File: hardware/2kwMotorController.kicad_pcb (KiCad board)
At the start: 4 copper layers, 170 x 98.5 mm, 415 parts, among them M3 MOUNTING_HOLE, M6 MOUNTING_HOLE, P1 CONN_01X02, P10 CONN_01_BRK, P11 CONN_01_M+, P12 CONN_01_M-, P13 CONN_01X02, P14 CONN_01X02, P15 CONN_01X04, P2 CONN_01X04, P3 CONN_01X09, P4 CONN_02X05, P5 CONN_01X03_UART, P6 CONN_01X03, P7 CONN_01X05, P8 CONN_01_V+, P9 CONN_01_V-, Q1 DMG4712SSS, Q10 PSMN021-100, Q2 DMG4712SSS, Q3 IRFP4468, Q5 IRFP4468, Q6 IRFP4468, Q7 IRFP4468, Q8 IRFP4468, Q9 IRFP4468, SW2 SW_PUSH, U1 LM358A, U10 MCP1501T-30E, U11 PDM1-S12-S3, U12 MIC5225-5.0, U13 TM4C1294KCPDT, U14 SN74LVCH2T45, U15 SN65HVD231D, U16 Si8045AA, U17 MIC4127, U18 MIC4127, U19 UCC27211, U2 LAH-100P, U20 Si8045AA, U21 74LVC1G17, U22 SN74LVCH2T45, U3 LOC110, U4 MCP6001, U5 ADA4805-1, U6 UCC27211, U7 MIC5225-5.0, U8 LT3471, U9 R-78E3.3-0.5, Y1 NX5032GA

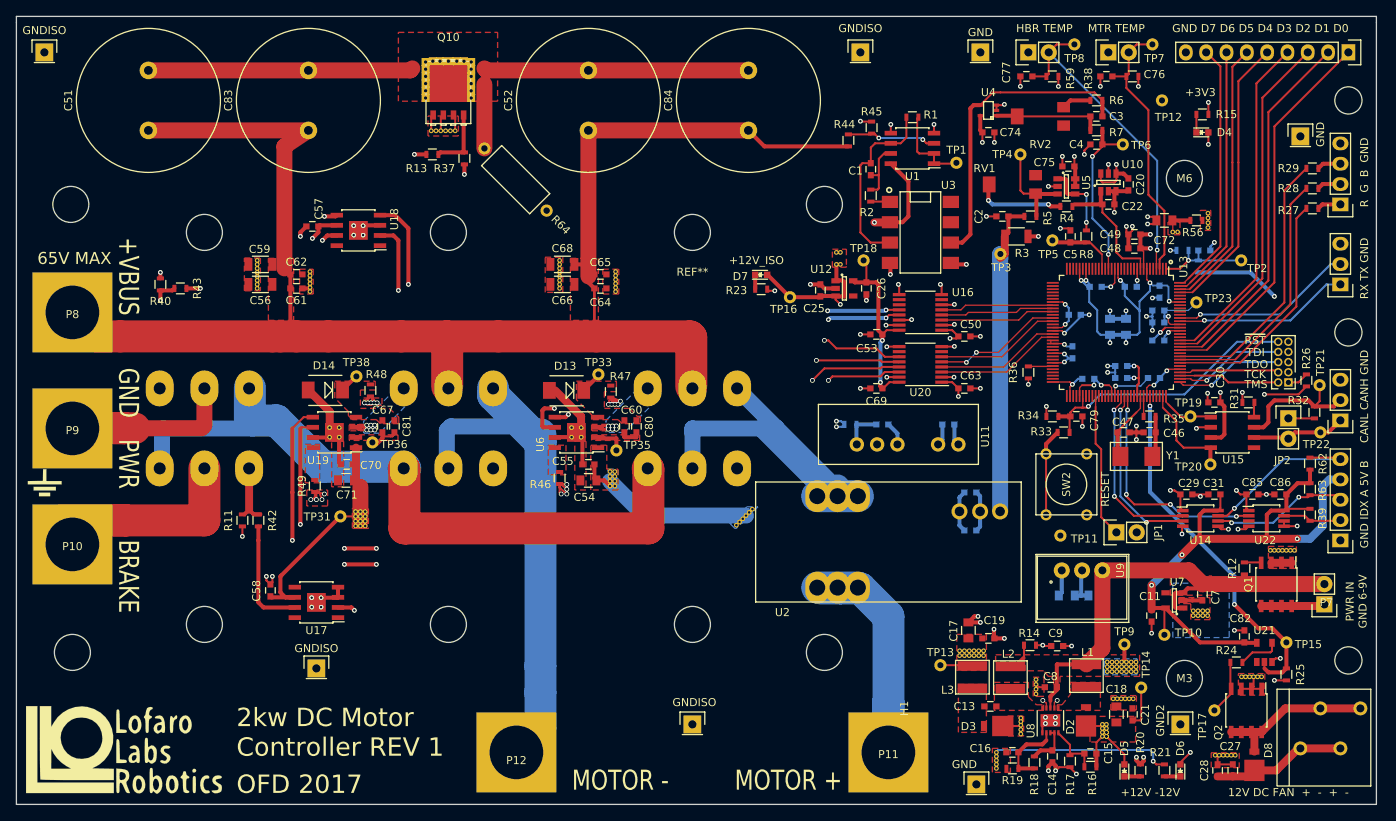
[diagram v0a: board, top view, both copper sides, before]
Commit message: minor hw changes to submit PCB Rev 1
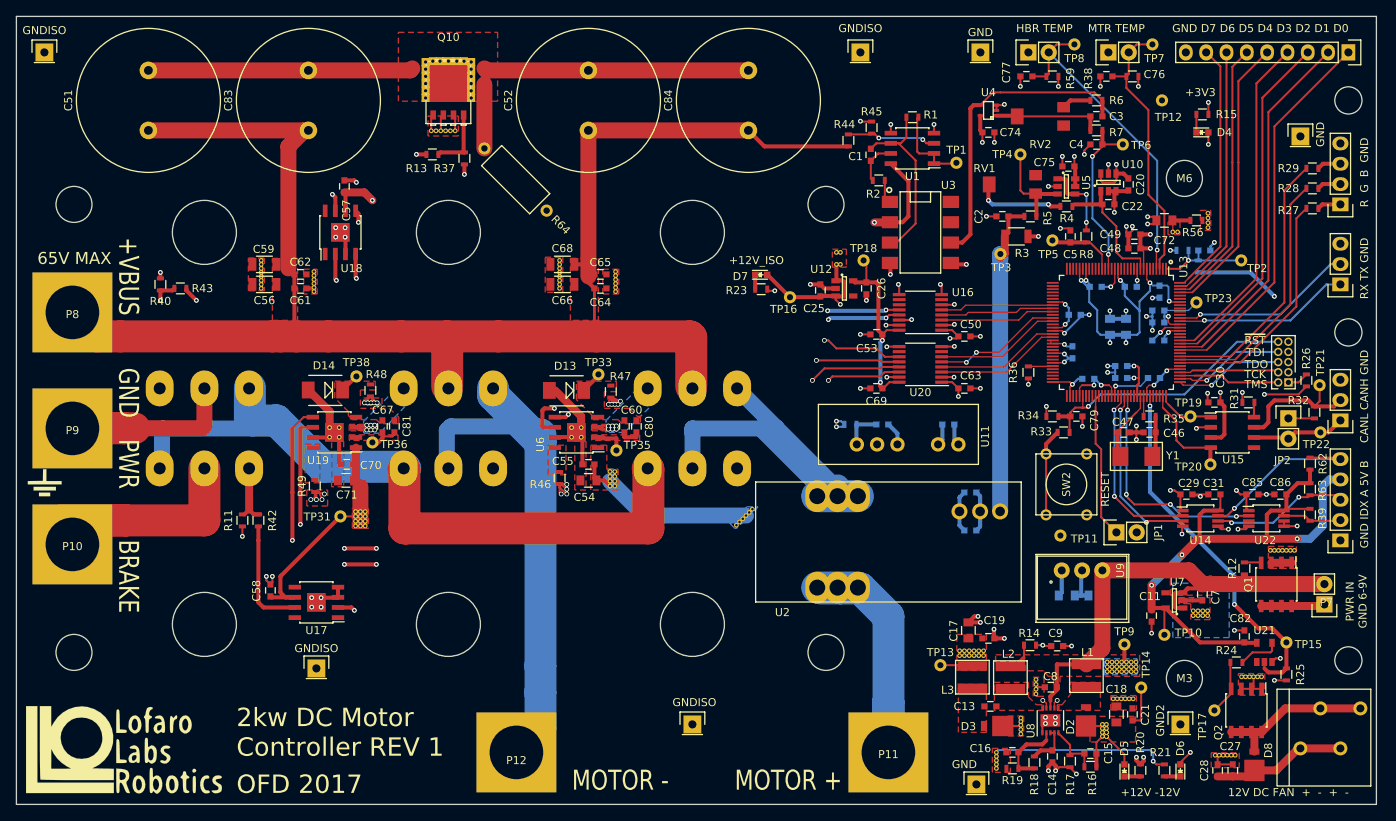
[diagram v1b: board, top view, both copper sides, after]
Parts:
- REF** (x6): footprint 2kwMotorController:M4-SCREW-HOLE -> 2kwMotorController:8MM_HOLE
- moved C57 6.40 mm to (74.5, 38.8), turned to 90 degrees
- moved U18 2.26 mm to (74.0, 44.5), turned to 90 degrees
- moved R2 2.15 mm to (141.3, 38.0), turned to 180 degrees
- moved C1 1.80 mm to (140.3, 34.8)
- moved C56 0.50 mm to (64.5, 51.0)
- moved C59 0.50 mm to (64.5, 48.5)
- moved C61 0.50 mm to (69.0, 51.5)
- moved C62 0.50 mm to (69.0, 49.8)
- moved REF**1111 0.50 mm to (70.7, 49.4)
- moved REF**1112 0.50 mm to (70.7, 49.9)
- moved REF**1113 0.50 mm to (70.7, 50.4)
- moved REF**1114 0.50 mm to (70.7, 50.9)
- moved REF**1115 0.50 mm to (70.7, 51.4)
- moved REF**1116 0.50 mm to (70.7, 51.9)
- moved REF**1111 0.50 mm to (64.1, 48.0)
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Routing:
- net Net-(R43-Pad1): track 22.9 -> 31.2 mm
- net Net-(R13-Pad1): track 19.5 -> 16.0 mm
- net /h-bridge/VBUS_ST_GD: track 73.7 -> 76.5 mm
- net +12V_ISO: track 275.8 -> 278.3 mm
- net Net-(C1-Pad1): track 7.59 -> 5.43 mm
- net /h-bridge/VBUS_EN_GD: track 74.0 -> 72.7 mm
- net Net-(C1-Pad2): track 23.5 -> 22.7 mm
- net Net-(R2-Pad1): track 2.41 -> 3.01 mm
- net GNDPWR: track 170.5 -> 170.0 mm
